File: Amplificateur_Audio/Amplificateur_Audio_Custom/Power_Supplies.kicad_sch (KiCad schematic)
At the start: 52 parts, among them J1001 PWR-IN, J1002 GND-IN

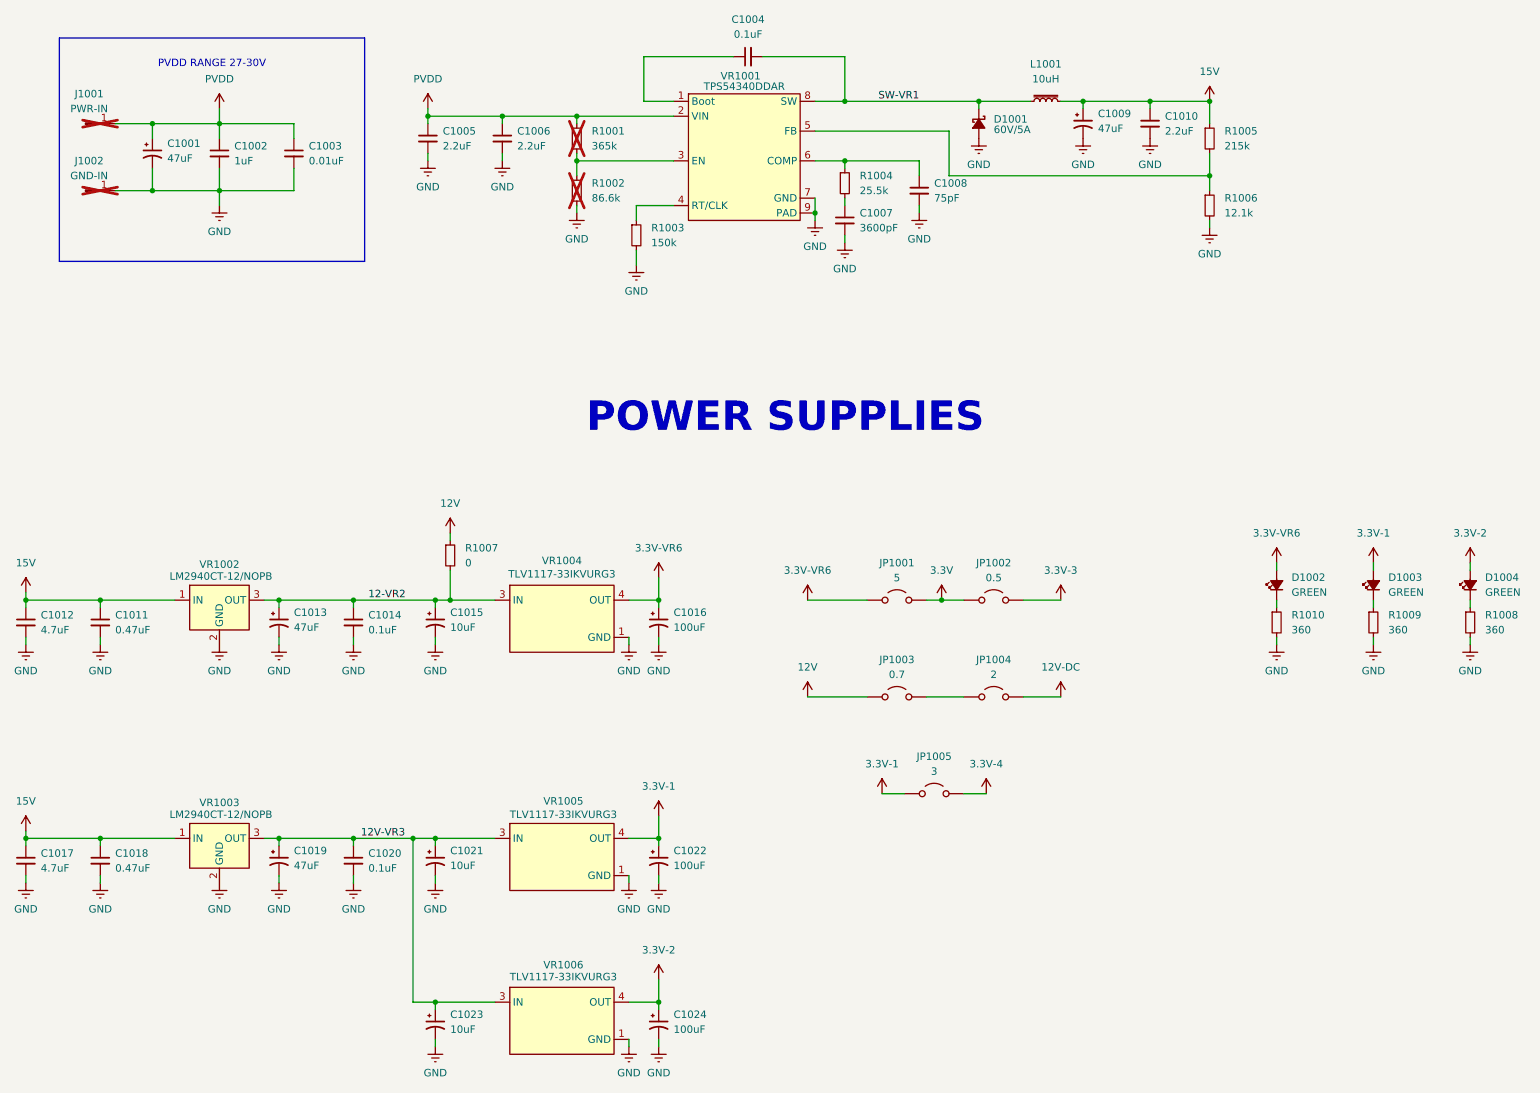
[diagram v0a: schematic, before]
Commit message: Assignation des composants et empreintes terminé
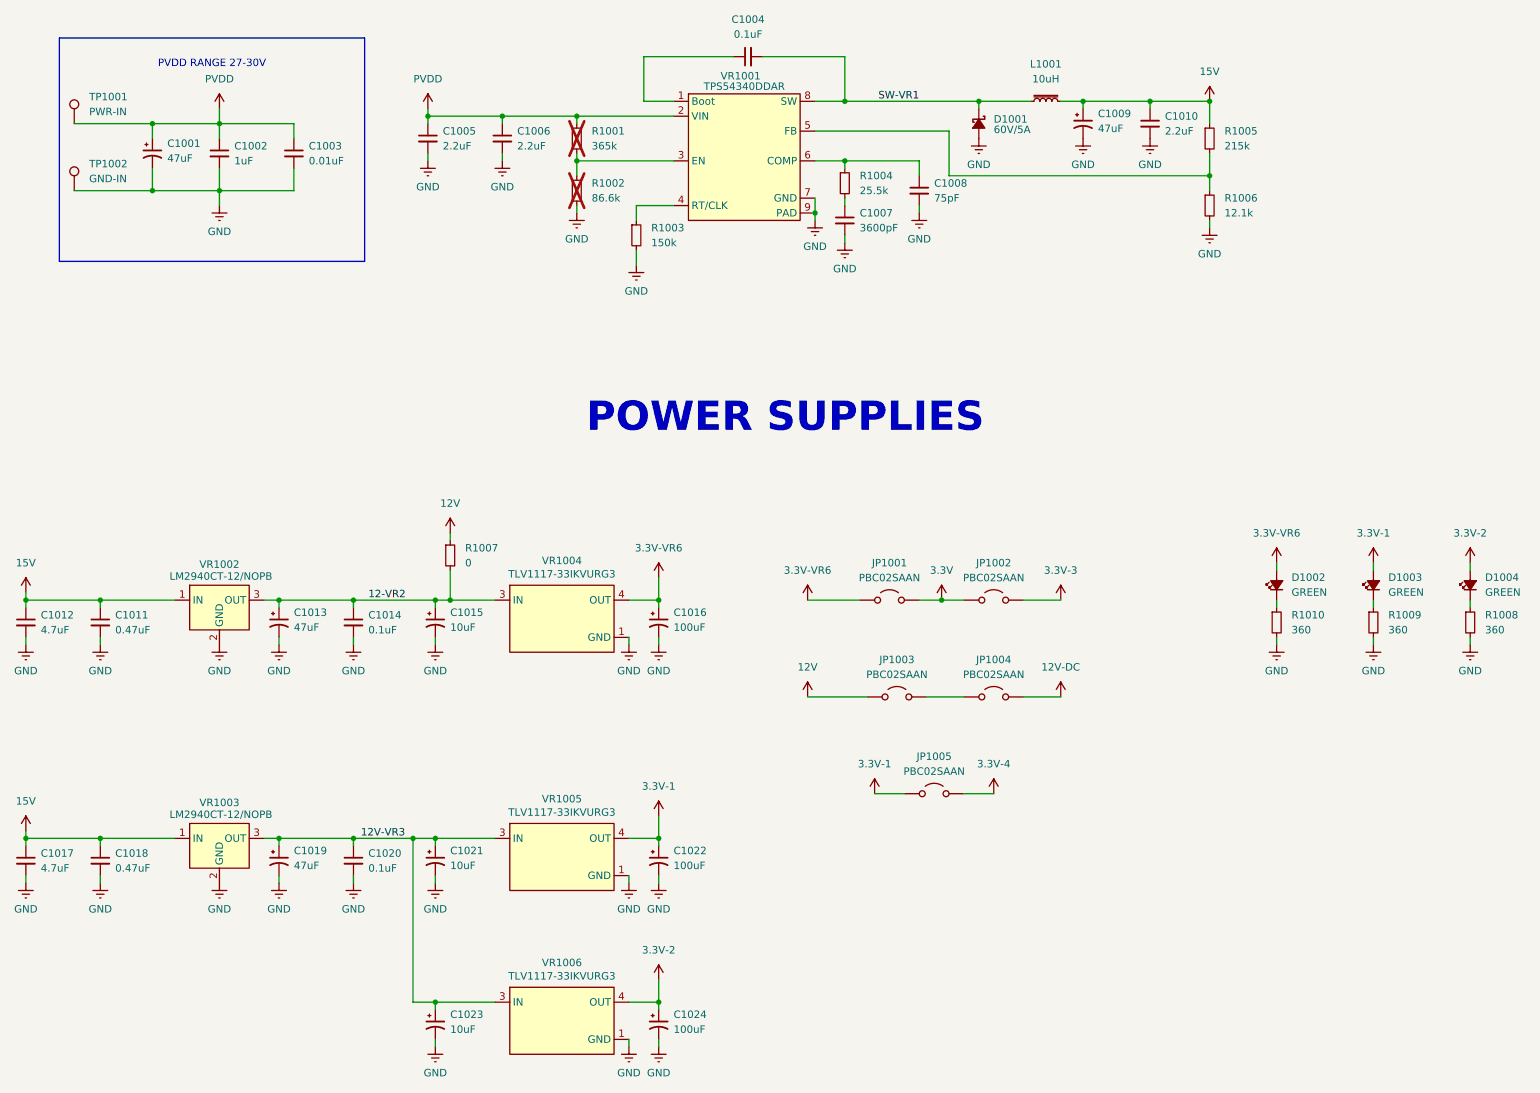
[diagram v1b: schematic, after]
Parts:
- removed J1001: PWR-IN, symbol Connector:Conn_01x01_Pin
- removed J1002: GND-IN, symbol Connector:Conn_01x01_Pin
- added TP1001: PWR-IN, symbol Connector:TestPoint
- added TP1002: GND-IN, symbol Connector:TestPoint
- C1001, C1009: footprint (none) -> Capacitor_SMD:CP_Elec_8x6.2
- C1002, C1003, C1004, C1007, C1008, C1011, C1014, C1018, C1020: footprint (none) -> Capacitor_SMD:C_0603_1608Metric_Pad1.08x0.95mm_HandSolder
- C1005, C1006, C1010: footprint (none) -> Capacitor_SMD:C_0805_2012Metric_Pad1.18x1.45mm_HandSolder
- C1012, C1017, R1007: footprint (none) -> Capacitor_SMD:C_1206_3216Metric_Pad1.33x1.80mm_HandSolder
- C1013, C1015, C1016, C1019, C1021, C1022, C1023, C1024: footprint (none) -> Capacitor_SMD:CP_Elec_6.3x5.8
- D1001: footprint (none) -> Diode_SMD:ST_D_SMC
- D1002, D1003, D1004: footprint (none) -> LED_SMD:LED_0805_2012Metric_Pad1.15x1.40mm_HandSolder
- JP1001: value 5 -> PBC02SAAN; footprint (none) -> NewLibrary:PBC02SAAN
- JP1002: value 0.5 -> PBC02SAAN; footprint (none) -> NewLibrary:PBC02SAAN
- JP1003: value 0.7 -> PBC02SAAN; footprint (none) -> NewLibrary:PBC02SAAN
- JP1004: value 2 -> PBC02SAAN; footprint (none) -> NewLibrary:PBC02SAAN
- JP1005: value 3 -> PBC02SAAN; footprint (none) -> NewLibrary:PBC02SAAN
- L1001: footprint (none) -> NewLibrary:WE-PD_1050P
- R1001, R1002, R1003, R1004, R1005, R1006: footprint (none) -> Resistor_SMD:R_0603_1608Metric_Pad0.98x0.95mm_HandSolder
- R1008, R1009, R1010: footprint (none) -> Capacitor_SMD:C_0402_1005Metric_Pad0.74x0.62mm_HandSolder
- VR1001: footprint (none) -> Package_SO:Texas_HTSOP-8-1EP_3.9x4.9mm_P1.27mm_EP2.95x4.9mm_Mask2.4x3.1mm_ThermalVias
- VR1002, VR1003: footprint (none) -> Package_TO_SOT_THT:TO-220-3_Horizontal_TabDown
- VR1004, VR1005, VR1006: footprint (none) -> Package_TO_SOT_SMD:TO-252-3_TabPin4
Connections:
- net GND: now also TP1002.1
- net PVDD: now also TP1001.1
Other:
- moved on the sheet: JP1001

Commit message: Ajout de point de test et début du routage
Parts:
- TP1001, TP1002: footprint (none) -> TestPoint:TestPoint_Pad_D1.5mm
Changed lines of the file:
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@@
 			)
 		)
-		(property "Footprint" ""
+		(property "Footprint" "TestPoint:TestPoint_Pad_D1.5mm"
 			(at 84.455 48.26 0)
 			(effects
@@
 			)
 		)
-		(property "Footprint" ""
+		(property "Footprint" "TestPoint:TestPoint_Pad_D1.5mm"
 			(at 84.455 59.69 0)
 			(effects

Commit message: Refactor : hierarchical template channels for multichannel routing
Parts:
- C1002, C1003, C1004, C1007, C1008, C1011, C1014, C1018, C1020: footprint Capacitor_SMD:C_0603_1608Metric_Pad1.08x0.95mm_HandSolder -> Capacitor_SMD:C_0603_1608Metric
- C1005, C1006, C1010: footprint Capacitor_SMD:C_0805_2012Metric_Pad1.18x1.45mm_HandSolder -> Capacitor_SMD:C_0805_2012Metric
- C1012, C1017: footprint Capacitor_SMD:C_1206_3216Metric_Pad1.33x1.80mm_HandSolder -> Capacitor_SMD:C_1206_3216Metric
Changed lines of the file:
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@@
 			)
 		)
-		(property "Footprint" "Capacitor_SMD:C_0603_1608Metric_Pad1.08x0.95mm_HandSolder"
+		(property "Footprint" "Capacitor_SMD:C_0603_1608Metric"
 			(at 210.82 64.77 0)
 			(effects
@@
 			)
 		)
-		(property "Footprint" "Capacitor_SMD:C_0805_2012Metric_Pad1.18x1.45mm_HandSolder"
+		(property "Footprint" "Capacitor_SMD:C_0805_2012Metric"
 			(at 139.7 50.8 0)
 			(effects
@@
 			)
 		)
-		(property "Footprint" "Capacitor_SMD:C_1206_3216Metric_Pad1.33x1.80mm_HandSolder"
+		(property "Footprint" "Capacitor_SMD:C_1206_3216Metric"
 			(at 71.12 133.35 0)
 			(effects
@@
 			)
 		)
-		(property "Footprint" "Capacitor_SMD:C_1206_3216Metric_Pad1.33x1.80mm_HandSolder"
+		(property "Footprint" "Capacitor_SMD:C_1206_3216Metric"
 			(at 71.12 173.99 0)
 			(effects
@@
 			)
 		)
-		(property "Footprint" "Capacitor_SMD:C_0603_1608Metric_Pad1.08x0.95mm_HandSolder"
+		(property "Footprint" "Capacitor_SMD:C_0603_1608Metric"
 			(at 104.14 53.34 0)
 			(effects
@@
 			)
 		)
-		(property "Footprint" "Capacitor_SMD:C_0805_2012Metric_Pad1.18x1.45mm_HandSolder"
+		(property "Footprint" "Capacitor_SMD:C_0805_2012Metric"
 			(at 152.4 50.8 0)
 			(effects
@@
 			)
 		)
-		(property "Footprint" "Capacitor_SMD:C_0603_1608Metric_Pad1.08x0.95mm_HandSolder"
+		(property "Footprint" "Capacitor_SMD:C_0603_1608Metric"
 			(at 127 133.35 0)
 			(effects
@@
 			)
 		)
-		(property "Footprint" "Capacitor_SMD:C_0603_1608Metric_Pad1.08x0.95mm_HandSolder"
+		(property "Footprint" "Capacitor_SMD:C_0603_1608Metric"
 			(at 194.31 36.83 0)
 			(effects
@@
 			)
 		)
-		(property "Footprint" "Capacitor_SMD:C_0603_1608Metric_Pad1.08x0.95mm_HandSolder"
+		(property "Footprint" "Capacitor_SMD:C_0603_1608Metric"
 			(at 223.52 59.69 0)
 			(effects
@@
 			)
 		)
-		(property "Footprint" "Capacitor_SMD:C_0603_1608Metric_Pad1.08x0.95mm_HandSolder"
+		(property "Footprint" "Capacitor_SMD:C_0603_1608Metric"
 			(at 83.82 173.99 0)
 			(effects
@@
 			)
 		)
-		(property "Footprint" "Capacitor_SMD:C_0603_1608Metric_Pad1.08x0.95mm_HandSolder"
+		(property "Footprint" "Capacitor_SMD:C_0603_1608Metric"
 			(at 127 173.99 0)
 			(effects
@@
 			)
 		)
-		(property "Footprint" "Capacitor_SMD:C_0603_1608Metric_Pad1.08x0.95mm_HandSolder"
+		(property "Footprint" "Capacitor_SMD:C_0603_1608Metric"
 			(at 116.84 53.34 0)
 			(effects
@@
 			)
 		)
-		(property "Footprint" "Capacitor_SMD:C_0603_1608Metric_Pad1.08x0.95mm_HandSolder"
+		(property "Footprint" "Capacitor_SMD:C_0603_1608Metric"
 			(at 83.82 133.35 0)
 			(effects
@@
 			)
 		)
-		(property "Footprint" "Capacitor_SMD:C_0805_2012Metric_Pad1.18x1.45mm_HandSolder"
+		(property "Footprint" "Capacitor_SMD:C_0805_2012Metric"
 			(at 262.89 48.26 0)
 			(effects
